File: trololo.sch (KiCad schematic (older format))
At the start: 103 parts, among them J1 10118194-0001LF, J10 Conn_02x12_Odd_Even, J11 Conn_02x02_Odd_Even, J13 PROTO1, J18 PROTO1, J2 10118194-0001LF, J3 RJ45_Amphenol_RJMG1BD3B8K1ANR, J4 Micro_SD_Card, J5 Screw_Terminal_01x06, J6 Conn_02x12_Odd_Even, J7 10118194-0001LF, J8 Screw_Terminal_01x02, J9 Conn_02x12_Odd_Even, SW1 RESET, SW2 PC13, U1 STM32H743VITx, U10 USBLC6-2SC6, U11 SN6505, U12 TCAN332, U13 ISL83483, U2 KSZ8081RNA, U3 ISO1050DUB, U4 ISO3082DW, U5 S25FL127SABMFI101, U6 AP63203, U7 USBLC6-2SC6, U8 STM32F042F6Px, U9 USBLC6-2SC6, Y1 8MHz, Y2 32.768KHz, Y3 25MHz

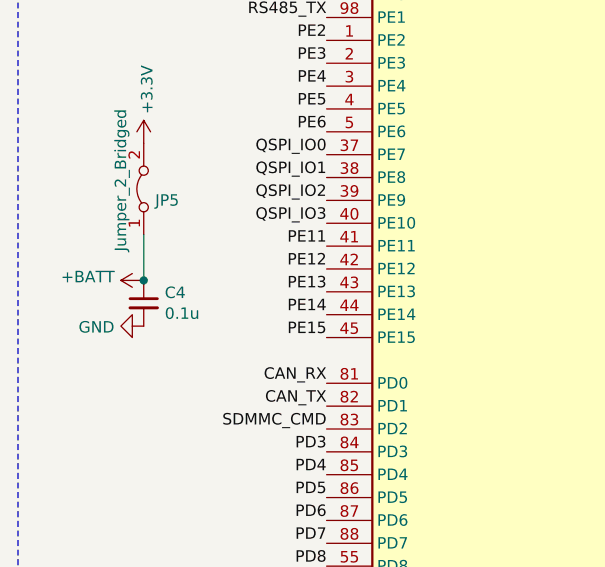
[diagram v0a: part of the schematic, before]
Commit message: More unprecie modifications
The log messages on this git sucks

Signed-off-by: Martin Ribelotta <martinribelotta@gmail.com>
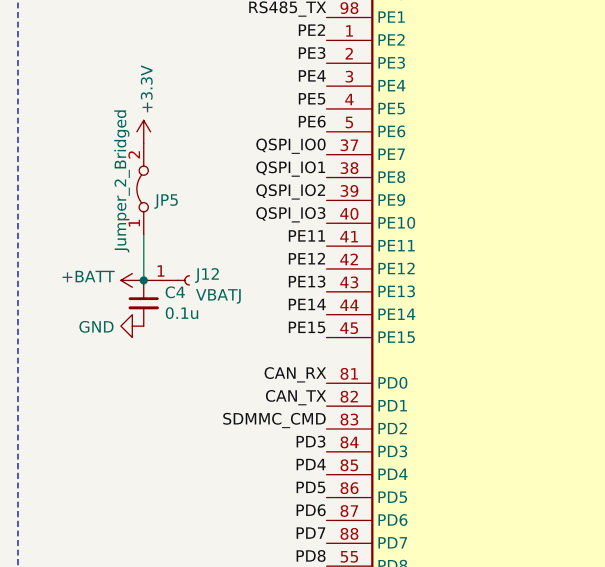
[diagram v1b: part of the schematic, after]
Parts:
- added J12: VBATJ, TestPoint:TestPoint_Loop_D1.80mm_Drill1.0mm_Beaded, symbol Connector:Conn_01x01_Female
- JP5: footprint Jumper:SolderJumper-2_P1.3mm_Open_RoundedPad1.0x1.5mm -> Jumper:SolderJumper-2_P1.3mm_Bridged_RoundedPad1.0x1.5mm
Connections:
- net +BATT: now also J12.1 (Pin_1)
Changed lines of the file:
@@
 	0    1    1    0
 $EndComp
-$Comp
-L Jumper:Jumper_2_Bridged JP5
-U 1 1 5CE929CB
-P 1100 4100
-F 0 "JP5" V 1050 4050 50  0000 R CNN
-F 1 "Jumper_2_Bridged" H 1450 4200 50  0000 R CNN
-F 2 "Jumper:SolderJumper-2_P1.3mm_Open_RoundedPad1.0x1.5mm" H 1100 4100 50  0001 C CNN
-F 3 "~" H 1100 4100 50  0001 C CNN
-	1    1100 4100
-	0    -1   -1   0
-$EndComp
+Connection ~ 1100 4500
 Wire Wire Line
 	1100 4300 1100 4500
-Connection ~ 1100 4500
 $Comp
 L power:+3.3V #PWR0184
@@
 	1    0    0    -1
 $EndComp
+$Comp
+L Jumper:Jumper_2_Bridged JP5
+U 1 1 5CE929CB
+P 1100 4100
+F 0 "JP5" V 1050 4050 50  0000 R CNN
+F 1 "Jumper_2_Bridged" H 1450 4200 50  0000 R CNN
+F 2 "Jumper:SolderJumper-2_P1.3mm_Bridged_RoundedPad1.0x1.5mm" H 1100 4100 50  0001 C CNN
+F 3 "~" H 1100 4100 50  0001 C CNN
+	1    1100 4100
+	0    -1   -1   0
+$EndComp
+$Comp
+L Connector:Conn_01x01_Female J12
+U 1 1 5CE79753
+P 1300 4500
+F 0 "J12" H 1328 4526 50  0000 L CNN
+F 1 "VBATJ" H 1328 4435 50  0000 L CNN
+F 2 "TestPoint:TestPoint_Loop_D1.80mm_Drill1.0mm_Beaded" H 1300 4500 50  0001 C CNN
+F 3 "~" H 1300 4500 50  0001 C CNN
+	1    1300 4500
+	1    0    0    -1
+$EndComp
